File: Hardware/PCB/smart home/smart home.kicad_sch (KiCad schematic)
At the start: 52 parts, among them M1 Fan, Q1 BC547C, Q10 BC547C, Q2 BC547C, Q3 BC547, Q4 BC547C, Q5 BC547C, Q6 BC547C, Q7 BC547C, Q8 BC547C, Q9 BC547C, SW1 SW_SPST, SW2 SW_SPST, SW3 SW_SPST, SW4 SW_Push, SW5 SW_Push, SW6 SW_Push

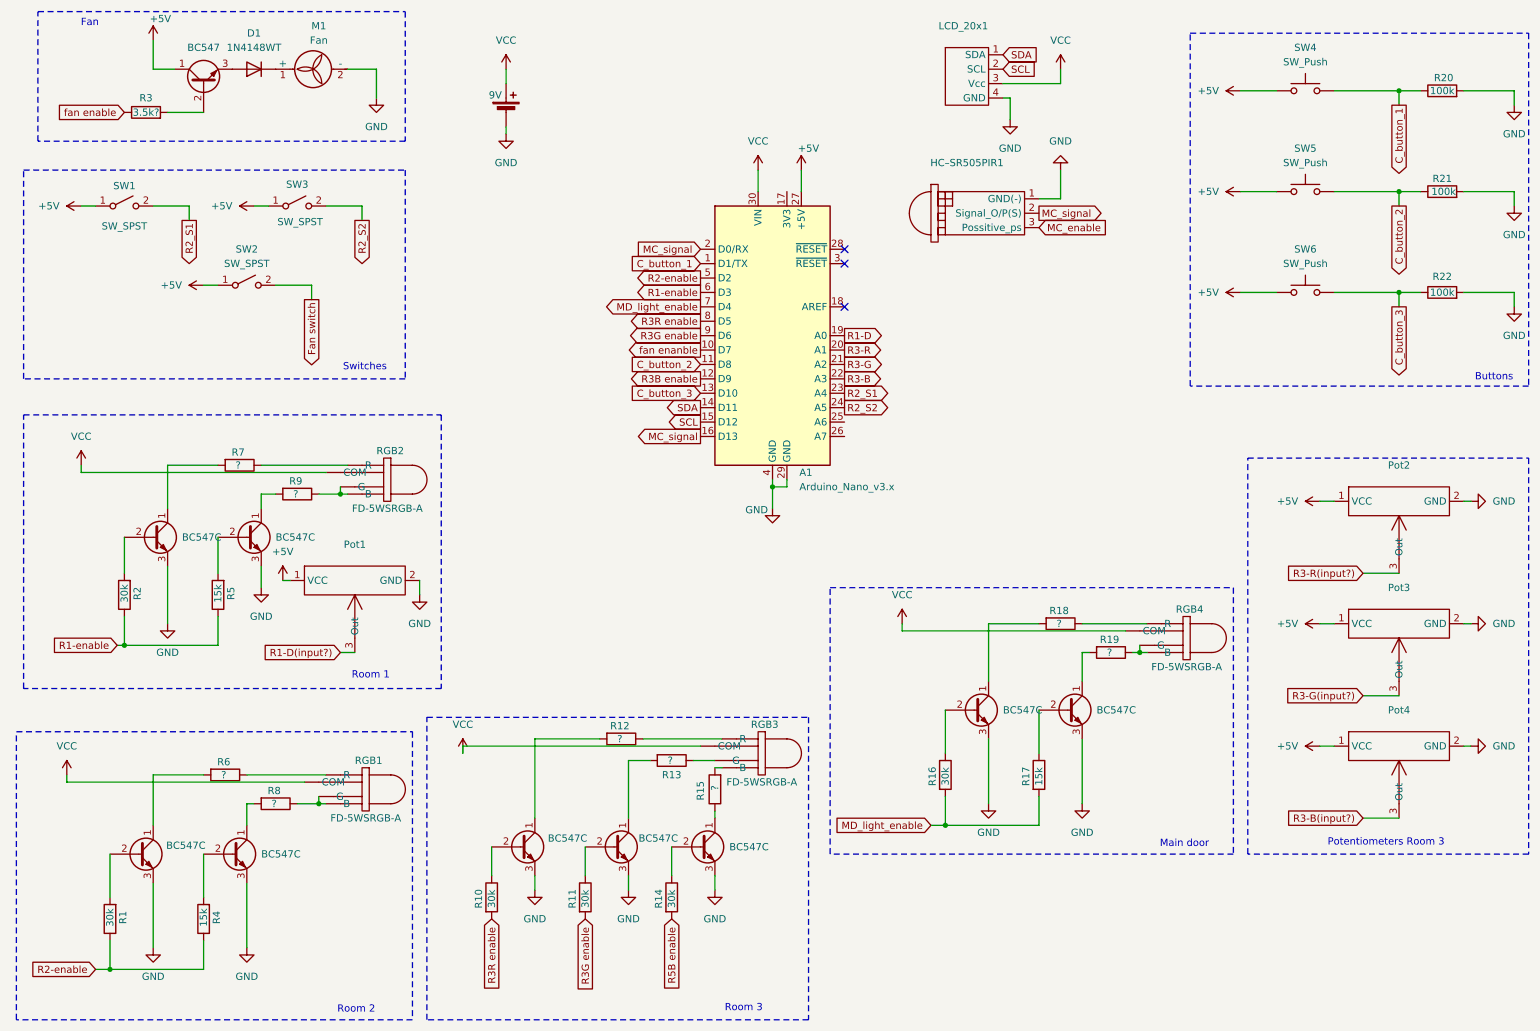
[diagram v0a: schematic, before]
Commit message: PCB should be right about done
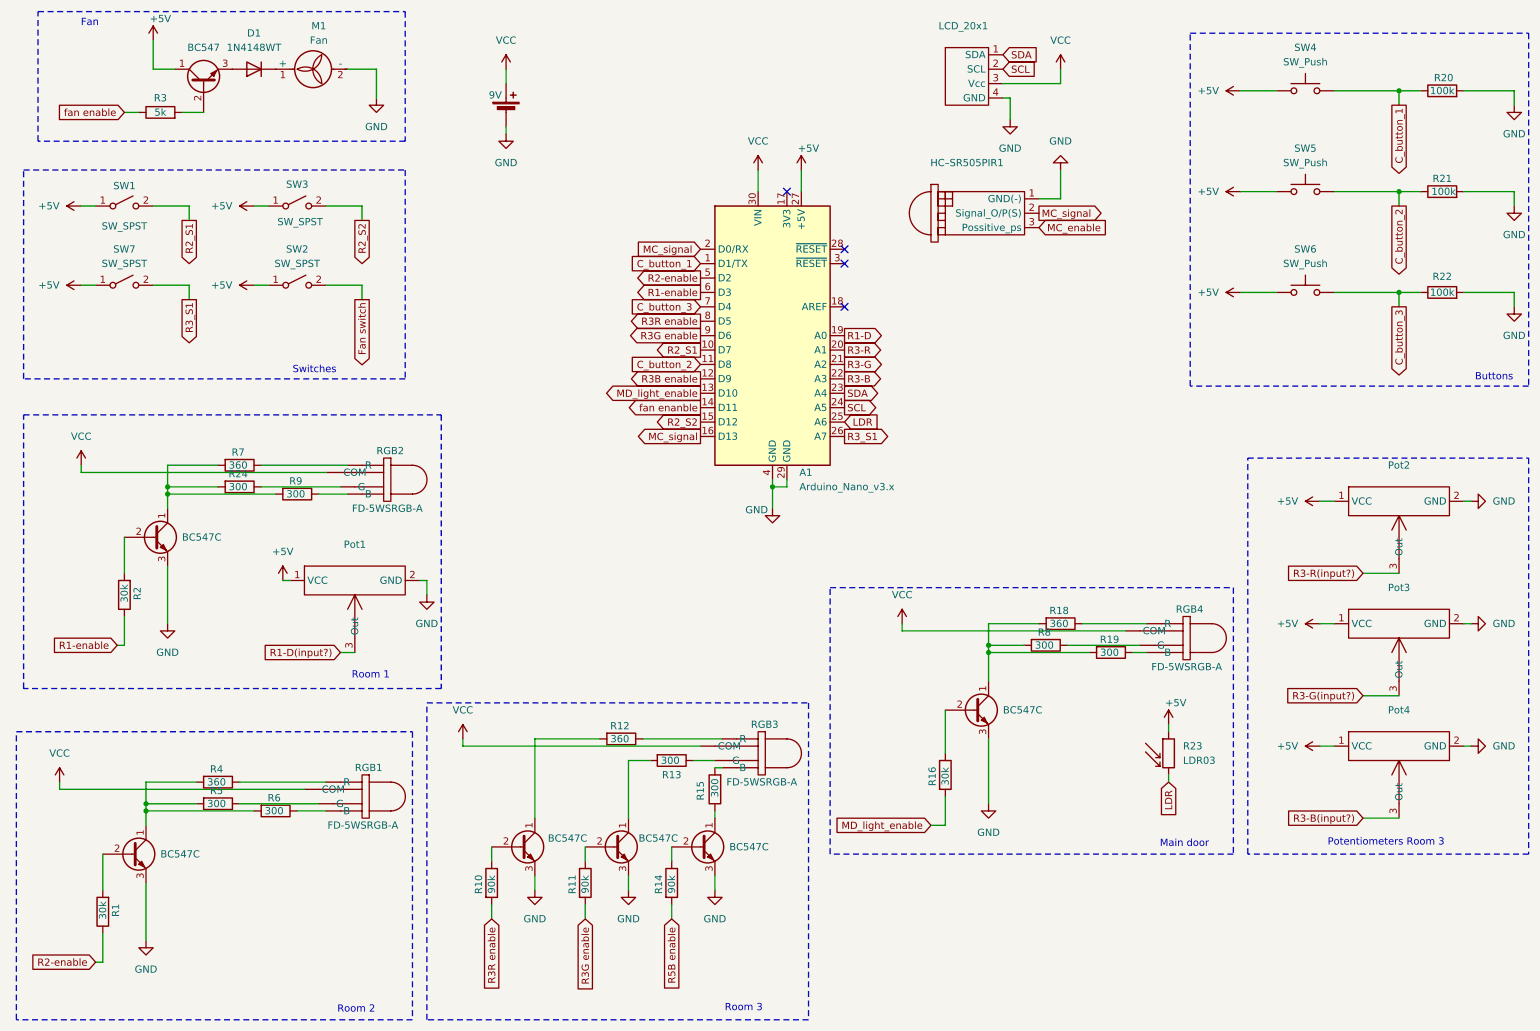
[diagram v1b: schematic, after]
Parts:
- removed Q10, Q4, Q5: BC547C, Package_TO_SOT_THT:TO-92_Inline, symbol Transistor_BJT:BC547
- removed R17: 15k, symbol Device:R
- added R23: LDR03, OptoDevice:R_LDR_10x8.5mm_P7.6mm_Vertical, symbol Sensor_Optical:LDR03
- added R24: 300, symbol Device:R
- added SW7: SW_SPST, symbol Switch:SW_SPST
- R10, R11, R14: value 30k -> 90k
- R12, R18, R7: value ? -> 360
- R13, R15, R19, R6, R8, R9: value ? -> 300
- R3: value 3.5k? -> 5k
- R4: value 15k -> 360
- R5: value 15k -> 300
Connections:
- net +5V: now also R23.1, SW7.1 (A)
- net C_button_3: now also A1.7 (D4); no longer A1.13 (D10)
- net MD_light_enable: now also A1.13 (D10); no longer A1.7 (D4)
- net R1-enable: no longer R5.1
- net R2-enable: no longer R4.1
- net R2_S1: now also A1.10 (D7); no longer A1.23 (A4)
- net R2_S2: now also A1.15 (D12); no longer A1.24 (A5)
- net SCL: now also A1.24 (A5); no longer A1.15 (D12)
- net SDA: now also A1.23 (A4); no longer A1.14 (D11)
- net fan enanble: now also A1.14 (D11); no longer A1.10 (D7)
- net at Q1.1 (C), R6.2: now also R4.2, R5.2
- net at Q2.1 (C), R7.2: now also R9.2, R24.2
- net at Q9.1 (C), R18.2: now also R19.2, R8.2
- net at R8.1: now also RGB4. (R); no longer RGB1. (R)
- net LDR: now reaches A1.25 (A6)
- net LDR: now also R23.2
- net R3_S1: now reaches A1.26 (A7)
- net R3_S1: now also SW7.2 (B)
- new net: R5.1, RGB1. (R)
- new net: R4.1, RGB1. (R)
- new net: R24.1, RGB2. (R)
- no-connect marks 3 -> 4
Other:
- moved on the sheet: R10, R11, R14, R3, SW2
